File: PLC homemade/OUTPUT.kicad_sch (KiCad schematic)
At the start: 14 parts, among them IC2 PCF8574DGVR, J3 M20-7820646, J4 M20-7820646, U7 SN74HCT14DR

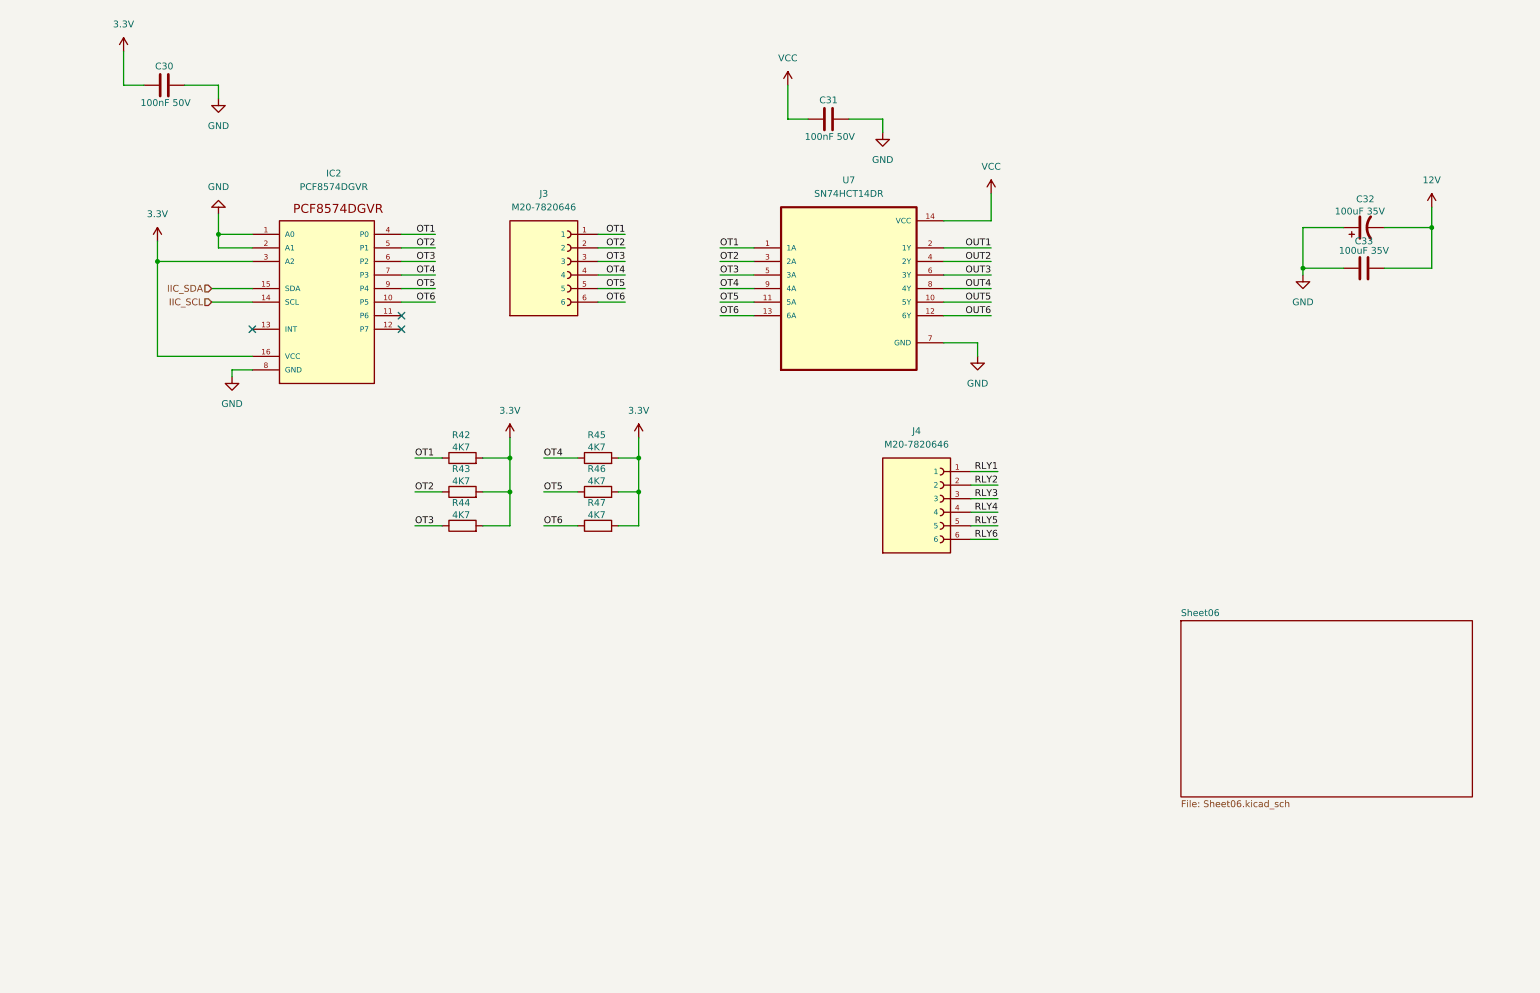
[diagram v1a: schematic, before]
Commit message: :tada: COMPLETED SHEET5
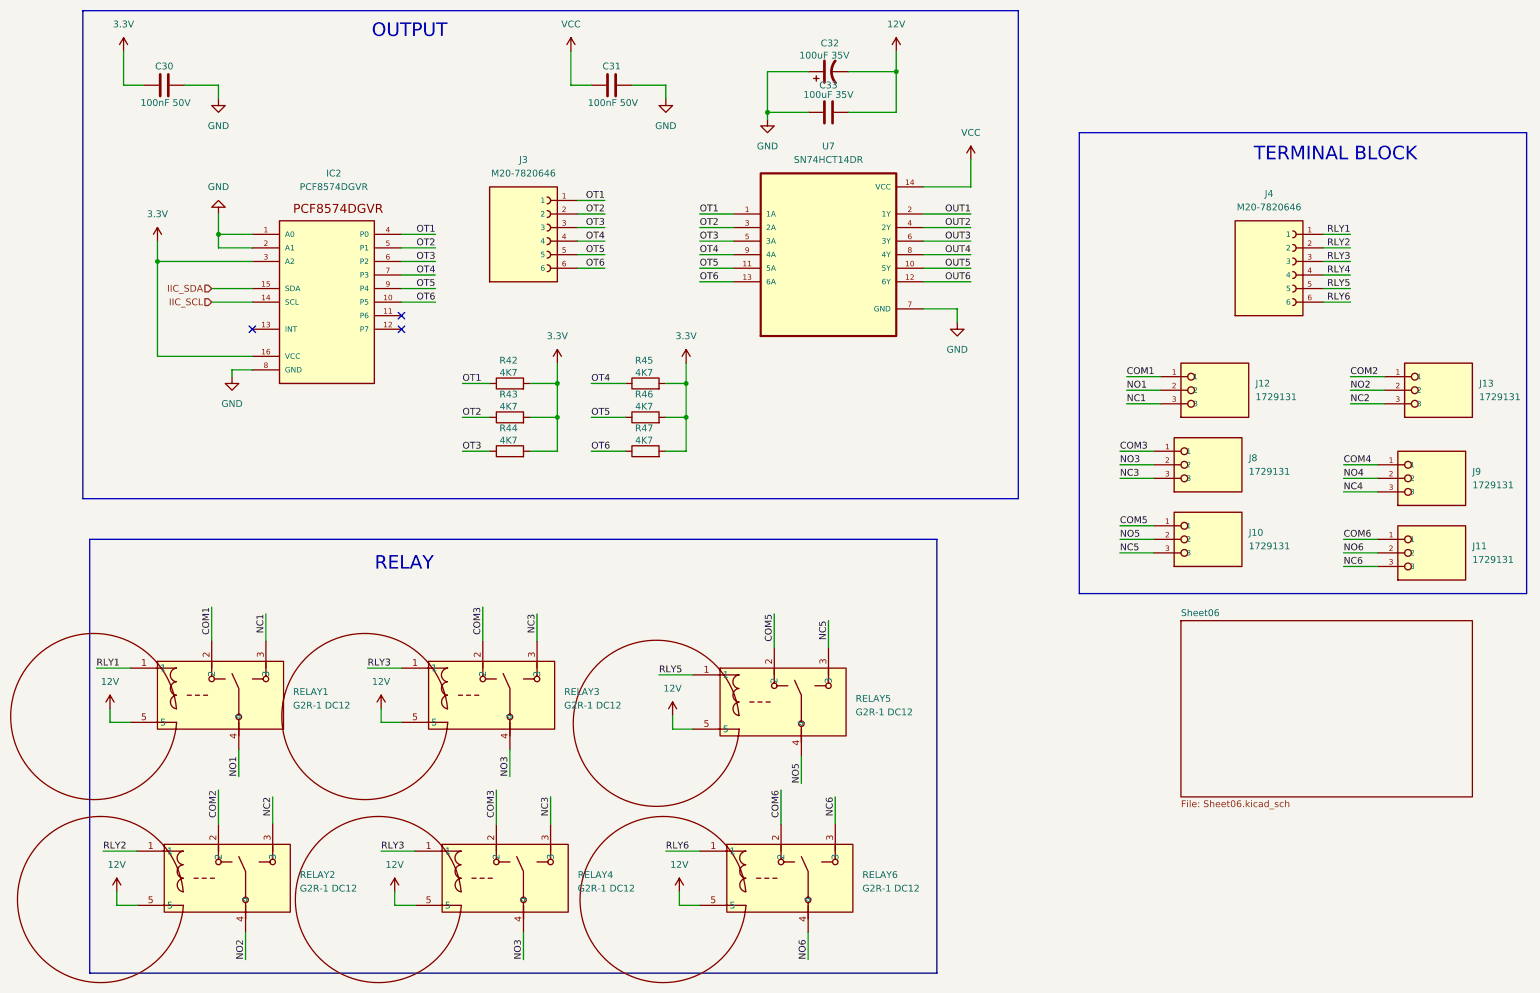
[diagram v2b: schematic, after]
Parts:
- added J10, J11, J12, J13, J8, J9: 1729131, 1729131:PHOENIX_1729131, symbol 1729131:1729131
- added RELAY1, RELAY2, RELAY3, RELAY4, RELAY5, RELAY6: G2R-1 DC12, G2R-1 DC12:RELAY-TH_G2R-1, symbol G2R-1 DC12:G2R-1DC12
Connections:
- net 12V: now also RELAY1.5, RELAY2.5, RELAY3.5, RELAY4.5, RELAY5.5, RELAY6.5
- net RLY1: now also RELAY1.1
- net RLY2: now also RELAY2.1
- net RLY3: now also RELAY3.1, RELAY4.1
- net RLY5: now also RELAY5.1
- net RLY6: now also RELAY6.1
- new net COM1: J12.1, RELAY1.2
- new net COM2: J13.1, RELAY2.2
- new net COM3: J8.1, RELAY3.2, RELAY4.2
- new net COM4: J9.1
- new net COM5: J10.1, RELAY5.2
- new net COM6: J11.1, RELAY6.2
- new net NC1: J12.3, RELAY1.3
- new net NC2: J13.3, RELAY2.3
- new net NC3: J8.3, RELAY3.3, RELAY4.3
- new net NC4: J9.3
- new net NC5: J10.3, RELAY5.3
- new net NC6: J11.3, RELAY6.3
- new net NO1: J12.2, RELAY1.4
- new net NO2: J13.2, RELAY2.4
- new net NO3: J8.2, RELAY3.4, RELAY4.4
- new net NO4: J9.2
- new net NO5: J10.2, RELAY5.4
- new net NO6: J11.2, RELAY6.4
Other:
- note added: "OUTPUT"
- note added: "RELAY"
- note added: "TERMINAL BLOCK"
- moved on the sheet: C31, C32, C33, J3, J4, R42, R43, R44, R45, R46, R47, U7
